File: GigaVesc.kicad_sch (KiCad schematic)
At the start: 35 parts, among them SW1 BOOT, SW3 RST, U1 STM32F405RGT6, U2 REF1933AIDDCT, X1 S5D8.000000A20F30T

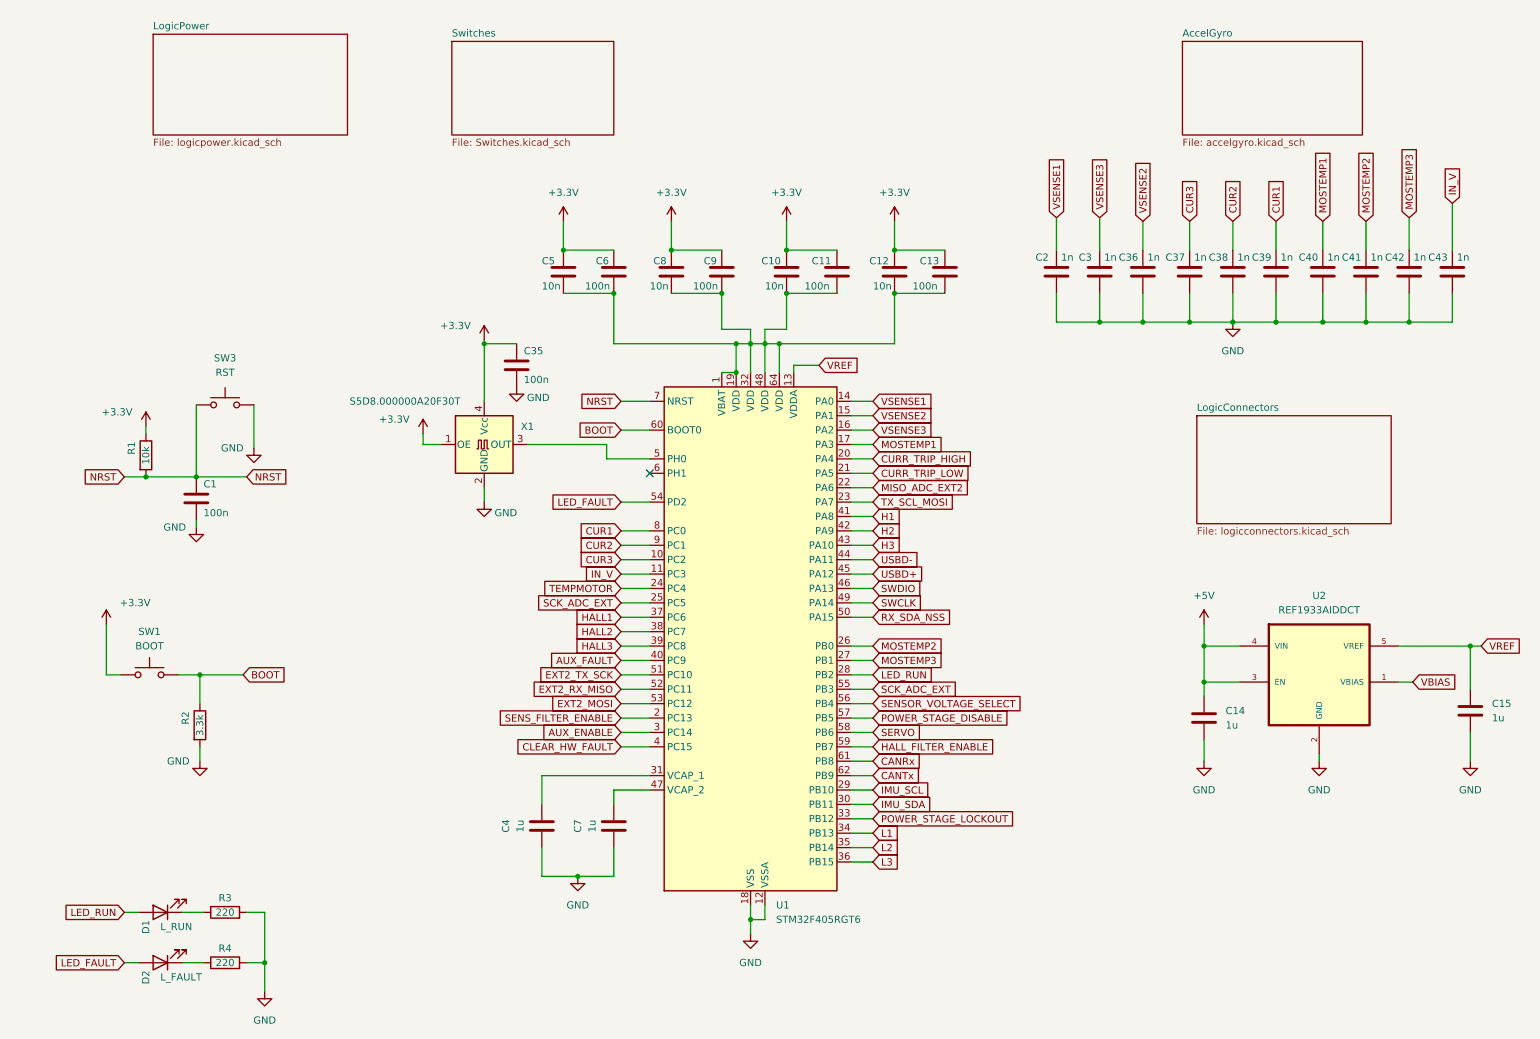
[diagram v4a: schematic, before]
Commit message: routed_again
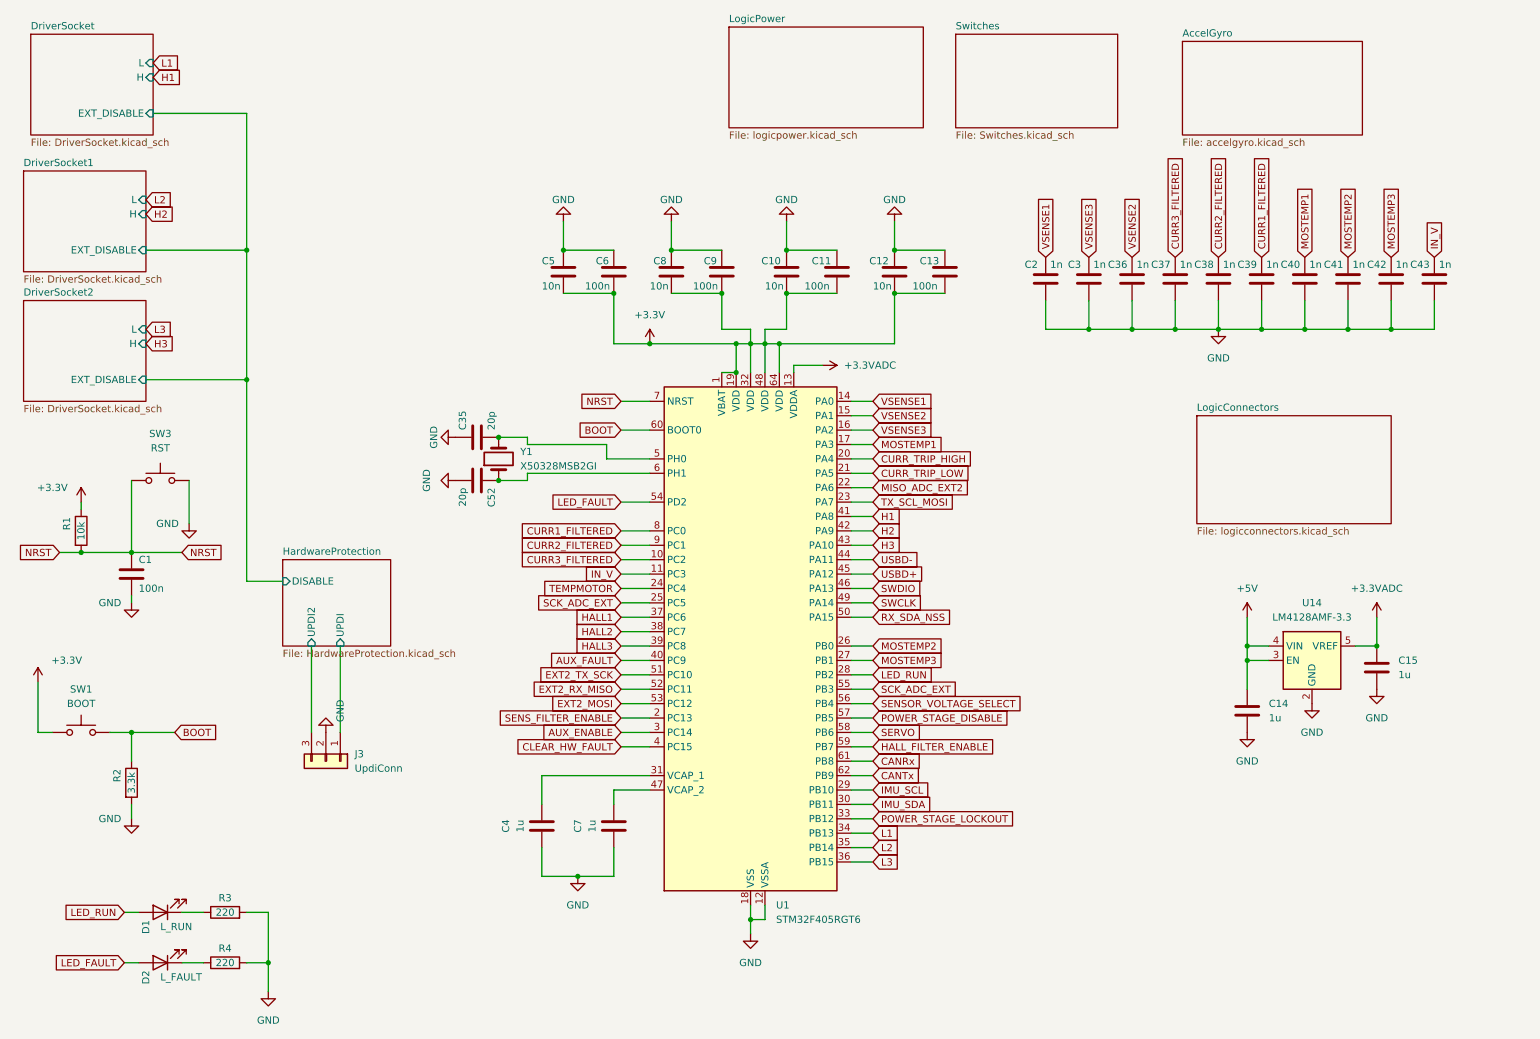
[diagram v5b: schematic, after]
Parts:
- removed U2: REF1933AIDDCT, Package_TO_SOT_SMD:SOT-23-5, symbol GigaVescSymbols:REF1933AIDDCT
- removed X1: S5D8.000000A20F30T, Crystal:Crystal_SMD_5032-4Pin_5.0x3.2mm, symbol Oscillator:SG-5032CCN
- added C52: 20p, Capacitor_SMD:C_0603_1608Metric, symbol Device:C
- added J3: UpdiConn, Connector_PinHeader_2.54mm:PinHeader_1x03_P2.54mm_Vertical, symbol Connector_Generic:Conn_01x03
- added U14: LM4128AMF-3.3, Package_TO_SOT_SMD:SOT-23-5, symbol Reference_Voltage:LM4128
- added Y1: X50328MSB2GI, Crystal:Crystal_SMD_5032-2Pin_5.0x3.2mm, symbol Device:Crystal
- C1: MPN C282732 -> C28233
- C10: MPN C83170 -> C1710
- C2: MPN C94121 -> C46653
- C35: value 100n -> 20p; footprint Capacitor_SMD:C_0805_2012Metric -> Capacitor_SMD:C_0603_1608Metric; MPN C282732 -> C1648
- D1: MPN C434435 -> C2297
- D2: MPN C131244 -> C84256
- R1: MPN C2930231 -> C17414
- R2: MPN C114531 -> C26010
- SW1, SW3: footprint Button_Switch_SMD:SW_SPST_Omron_B3FS-100xP -> Button_Switch_SMD:SW_Tactile_SPST_NO_Straight_CK_PTS636Sx25SMTRLFS; MPN C271750 -> C329185
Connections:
- net +3.3V: now also C10.2, C11.2, C12.2, C13.2, C5.2, C6.2, C8.2, C9.2, U1.1 (VBAT), U1.19 (VDD), U1.32 (VDD), U1.48 (VDD), U1.64 (VDD); no longer C10.1, C11.1, C12.1, C13.1, C35.1, C5.1, C6.1, C8.1, C9.1
- net +5V: now also U14.3 (EN), U14.4 (VIN)
- net GND: now also C10.1, C11.1, C12.1, C13.1, C35.1, C5.1, C6.1, C8.1, C9.1, C52.2, J3.2 (Pin_2), U14.2 (GND); no longer C35.2
- net at U1.5 (PH0): now also C35.2, Y1.2
- net at U1.6 (PH1): now also C52.1, Y1.1
- net CUR1 renamed CURR1_FILTERED
- net CUR2 renamed CURR2_FILTERED
- net CUR3 renamed CURR3_FILTERED
- net VREF renamed +3.3VADC
- net +3.3VADC: now also U14.5 (VREF)
- new net HardwareProtection/UPDI: J3.1 (Pin_1)
- new net HardwareProtection/UPDI2: J3.3 (Pin_3)
- no-connect marks 1 -> 0
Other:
- added sheet DriverSocket (DriverSocket.kicad_sch)
- added sheet DriverSocket1 (DriverSocket.kicad_sch)
- added sheet DriverSocket2 (DriverSocket.kicad_sch)
- added sheet HardwareProtection (HardwareProtection.kicad_sch)
- moved on the sheet: C1, C14, C15, C2, C3, C35, C36, C37, C38, C39, C40, C41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

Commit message: pre-final
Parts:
- J3: JLCPosOffset (none) -> 2.54,0; JLCRotOffset (none) -> -90
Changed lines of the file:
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@@
+      (effects (font (size 1.27 1.27)) hide)
+    )
+    (property "JLCRotOffset" "-90" (at 71.12 147.32 90)
+      (effects (font (size 1.27 1.27)) hide)
+    )
+    (property "JLCPosOffset" "2.54,0" (at 71.12 147.32 90)
       (effects (font (size 1.27 1.27)) hide)
     )
